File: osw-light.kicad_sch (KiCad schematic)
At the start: 54 parts, among them J1 Conn_02x12_Odd_Even, J2 Conn_01x06, Q1 2N7002, U1 RV-3028-C7, U2 LIS2DTW12TR, U3 ESP32-PICO-D4, U4 XC6209, U5 BQ51050BRHL, U6 XC6209

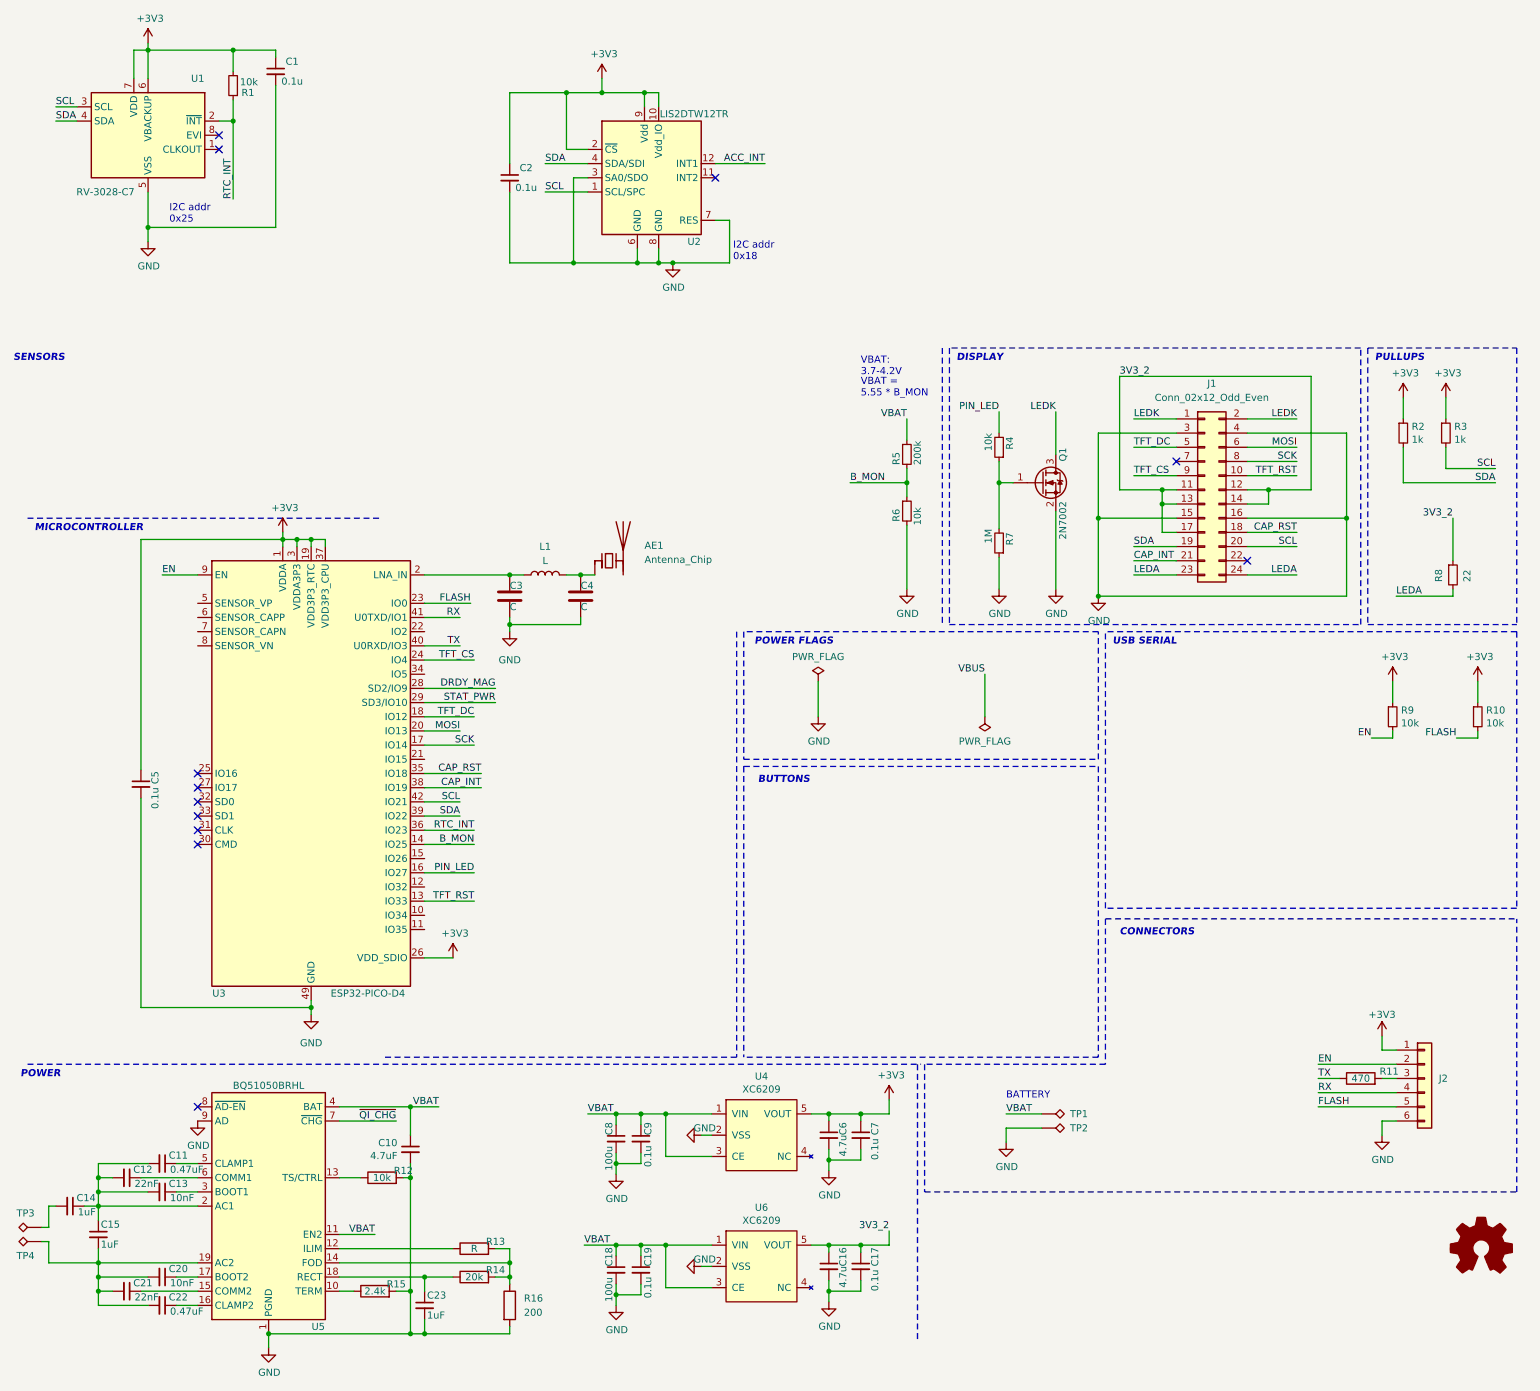
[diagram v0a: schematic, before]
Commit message: Near finished with Rev2 Design
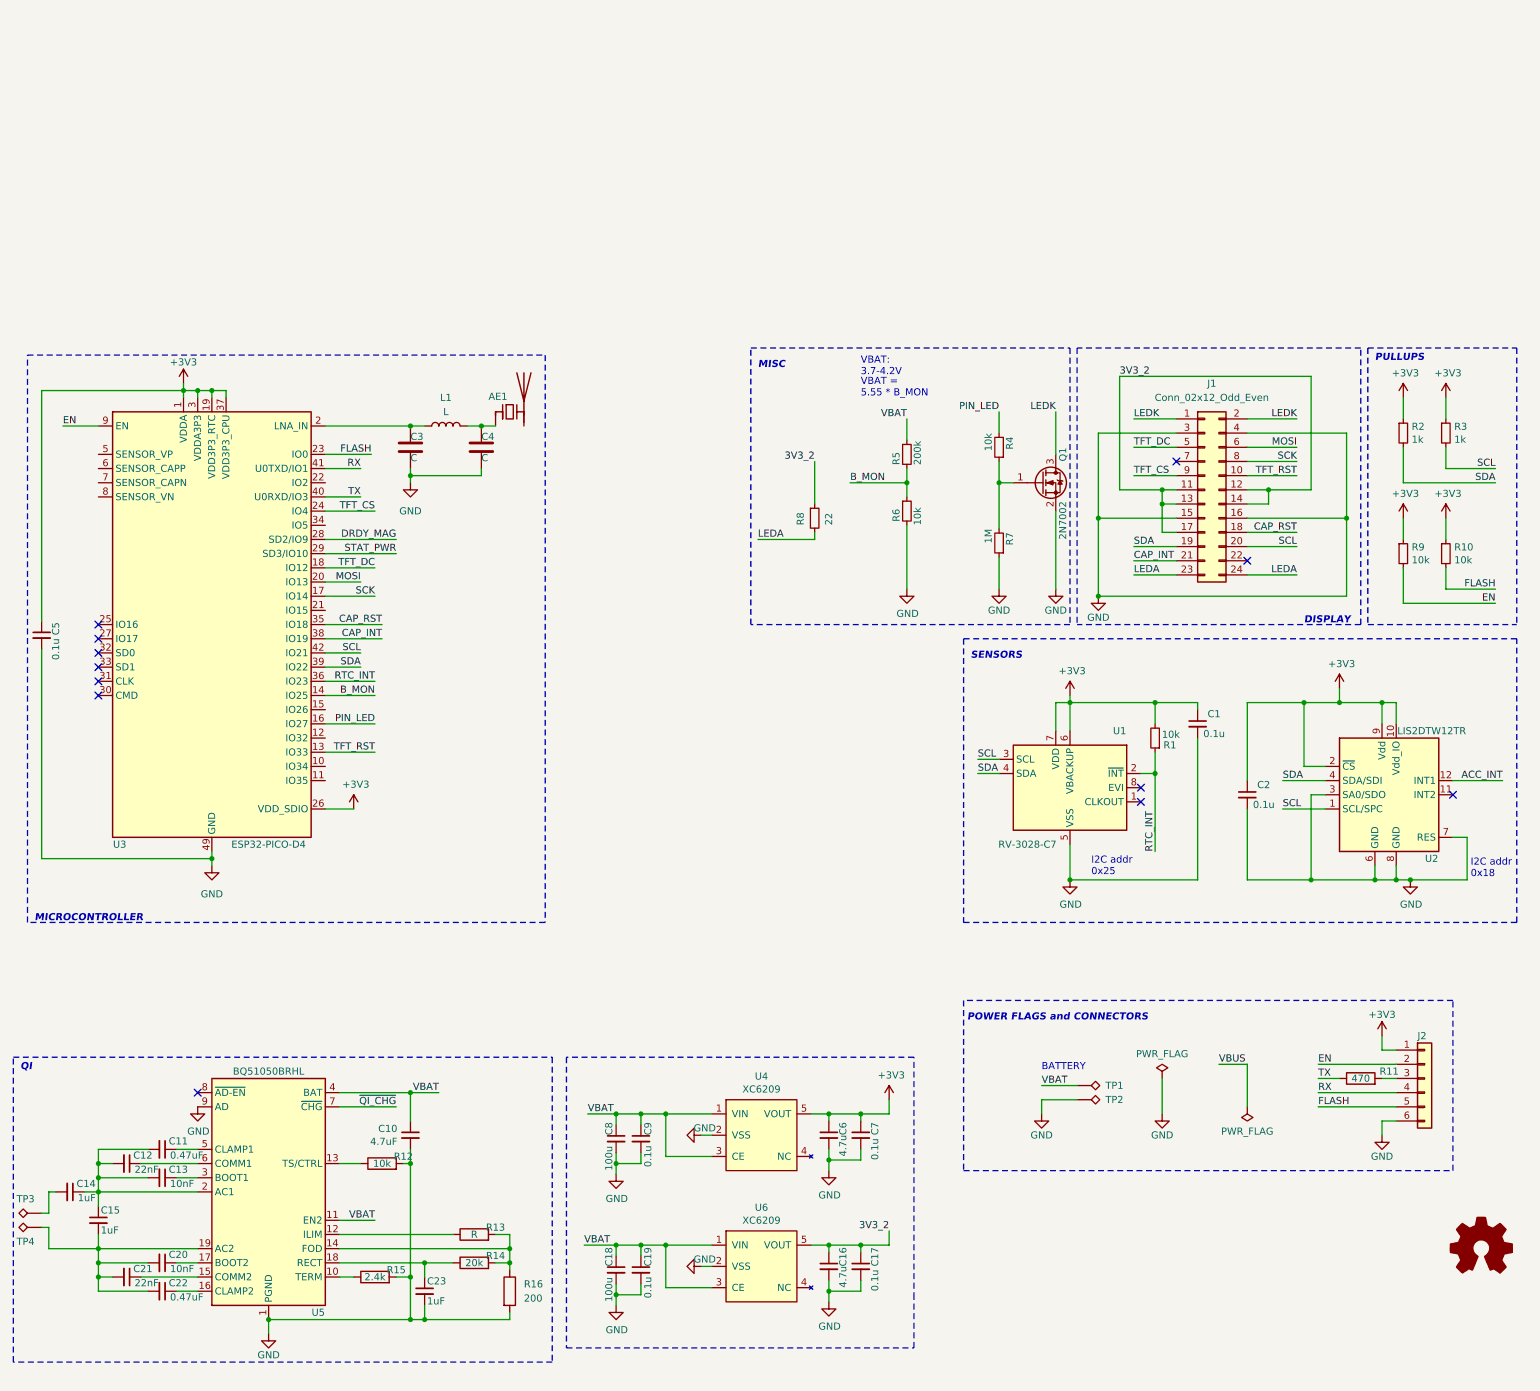
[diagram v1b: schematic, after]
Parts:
- C10, C14, C15: footprint Capacitor_SMD:C_0603_1608Metric -> Capacitor_SMD:C_0805_2012Metric
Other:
- note added: "MISC"
- note added: "POWER FLAGS and CONNECTORS"
- note added: "QI"
- note removed: "BUTTONS"
- note removed: "CONNECTORS"
- note removed: "POWER"
- note removed: "POWER FLAGS"
- note removed: "USB SERIAL"
- moved on the sheet: AE1, C1, C10, C11, C12, C13, C14, C15, C2, C20, C21, C22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
